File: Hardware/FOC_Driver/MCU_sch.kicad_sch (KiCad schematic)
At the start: 1 part, among them U1 STM32G431CBUx

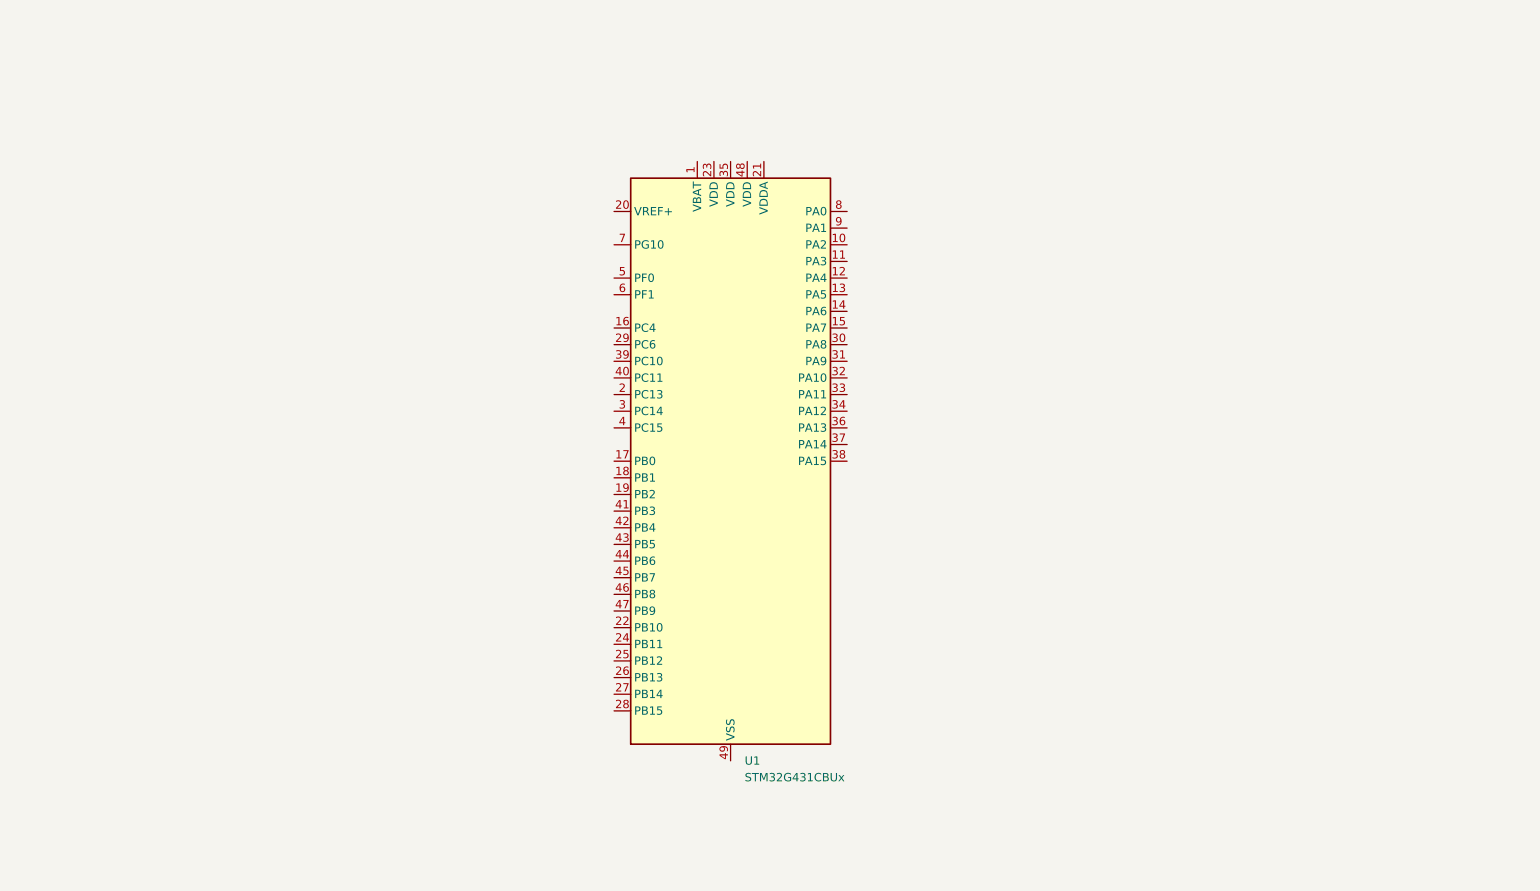
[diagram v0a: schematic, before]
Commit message: Schematic update and Firmware folder
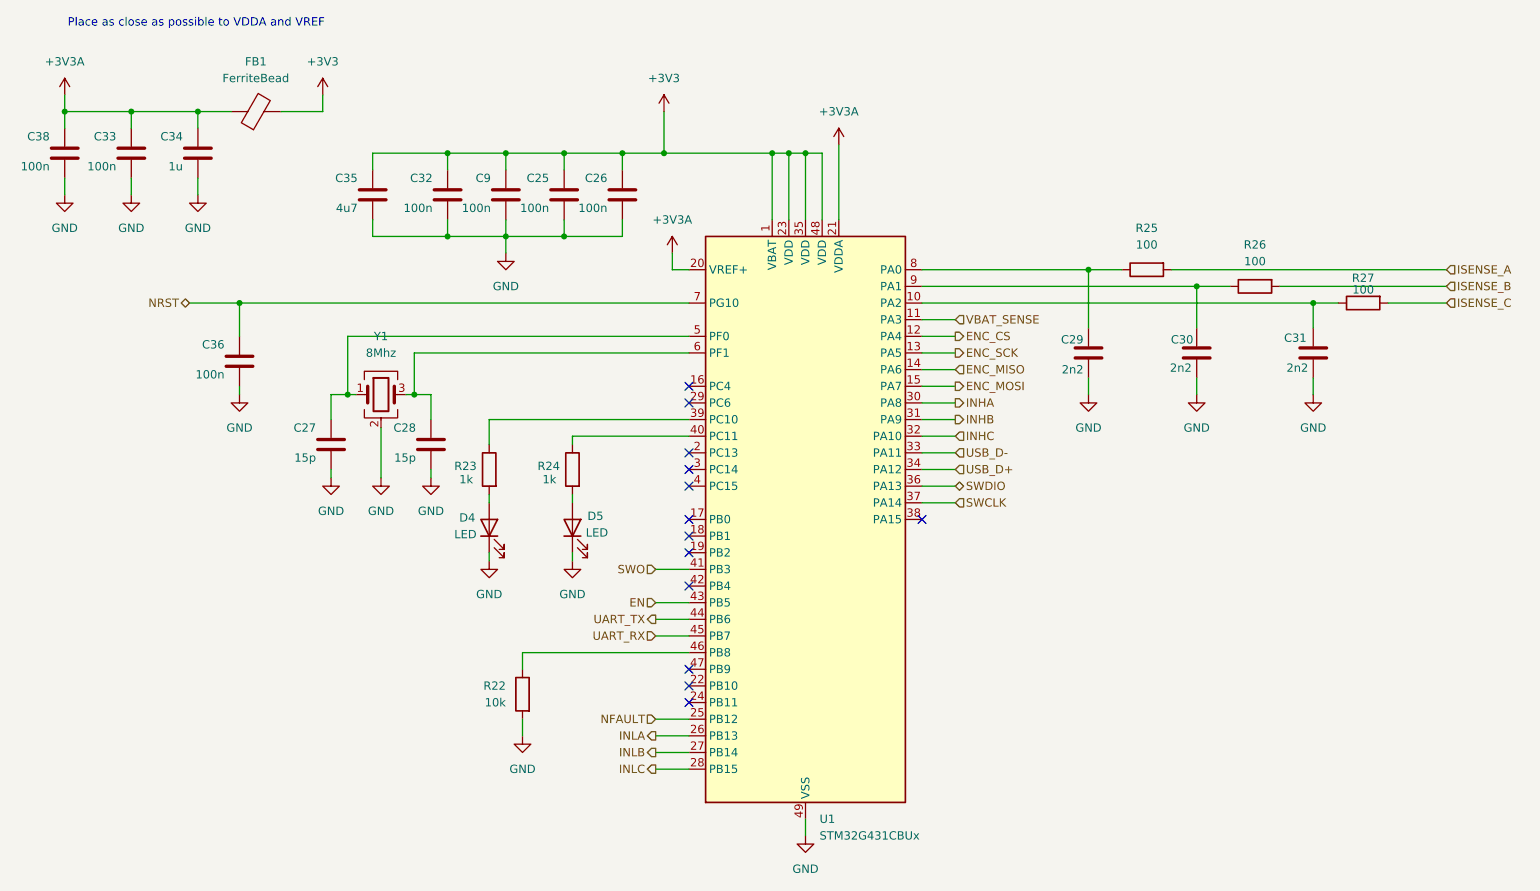
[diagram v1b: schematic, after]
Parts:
- added C25, C26, C32, C33, C36, C38, C9: 100n, symbol Device:C
- added C27, C28: 15p, symbol Device:C
- added C29, C30, C31: 2n2, symbol Device:C
- added C34: 1u, symbol Device:C
- added C35: 4u7, symbol Device:C
- added D4, D5: LED, symbol Device:LED
- added FB1: FerriteBead, symbol Device:FerriteBead
- added R22: 10k, symbol Device:R
- added R23, R24: 1k, symbol Device:R
- added R25, R26, R27: 100, symbol Device:R
- added Y1: 8Mhz, symbol Device:Crystal_GND24
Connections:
- net +3V3: now reaches U1.1 (VBAT)
- net +3V3: now also U1.23 (VDD), U1.35 (VDD), U1.48 (VDD), C25.2, C26.2, C32.2, C35.2, C9.2, FB1.2
- net at U1.10 (PA2): now also C31.2, R27.1
- net VBAT_SENSE: now reaches U1.11 (PA3)
- net ENC_CS: now reaches U1.12 (PA4)
- net ENC_SCK: now reaches U1.13 (PA5)
- net ENC_MISO: now reaches U1.14 (PA6)
- net ENC_MOSI: now reaches U1.15 (PA7)
- net +3V3A: now reaches U1.20 (VREF+)
- net +3V3A: now also U1.21 (VDDA), C33.2, C34.2, C38.2, FB1.1
- net NFAULT: now reaches U1.25 (PB12)
- net INLA: now reaches U1.26 (PB13)
- net INLB: now reaches U1.27 (PB14)
- net INLC: now reaches U1.28 (PB15)
- net INHA: now reaches U1.30 (PA8)
- net INHB: now reaches U1.31 (PA9)
- net INHC: now reaches U1.32 (PA10)
- net USB_D-: now reaches U1.33 (PA11)
- net USB_D+: now reaches U1.34 (PA12)
- net SWDIO: now reaches U1.36 (PA13)
- net SWCLK: now reaches U1.37 (PA14)
- net at U1.39 (PC10): now also R23.1
- net at U1.40 (PC11): now also R24.1
- net SWO: now reaches U1.41 (PB3)
- net EN: now reaches U1.43 (PB5)
- net UART_TX: now reaches U1.44 (PB6)
- net UART_RX: now reaches U1.45 (PB7)
- net at U1.46 (PB8): now also R22.1
- net GND: now reaches U1.49 (VSS)
- net GND: now also C25.1, C26.1, C27.1, C28.1, C29.1, C30.1, C31.1, C32.1, C33.1, C34.1, C35.1, C36.1, C38.1, C9.1, D4.1 (K), D5.1 (K), R22.2, Y1.2 (G), Y1.4 (G)
- net at U1.5 (PF0): now also C27.2, Y1.1
- net at U1.6 (PF1): now also C28.2, Y1.3
- net NRST: now reaches U1.7 (PG10)
- net NRST: now also C36.2
- net at U1.8 (PA0): now also C29.2, R25.1
- net at U1.9 (PA1): now also C30.2, R26.1
- new net: D5.2 (A), R24.2
- new net: D4.2 (A), R23.2
- new net ISENSE_A: R25.2
- new net ISENSE_B: R26.2
- new net ISENSE_C: R27.2
- no-connect marks 0 -> 13
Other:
- note added: "Place as close as possible to VDDA and VREF"
- moved on the sheet: U1
